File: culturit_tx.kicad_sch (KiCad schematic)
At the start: 0 parts

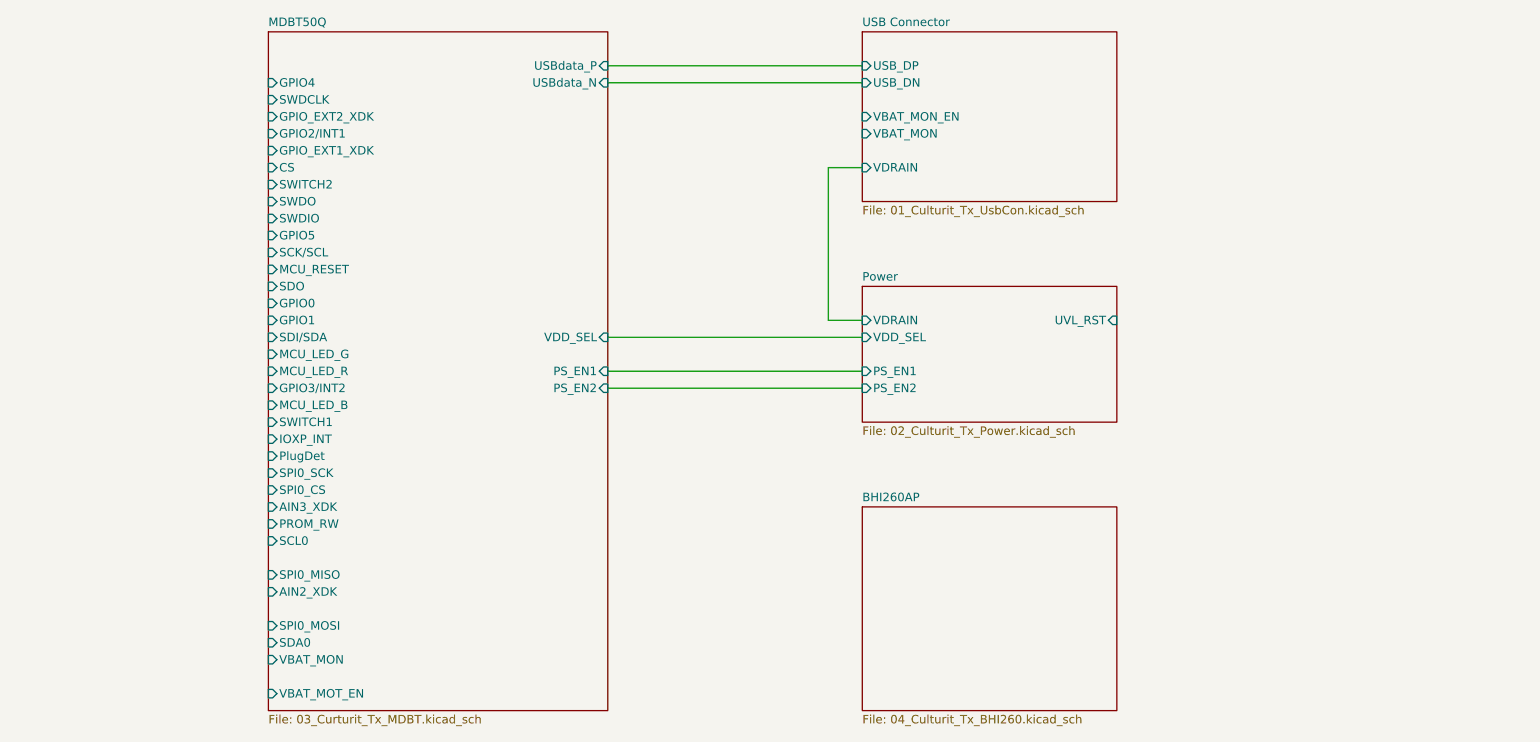
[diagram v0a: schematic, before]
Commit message: 2022-08-10
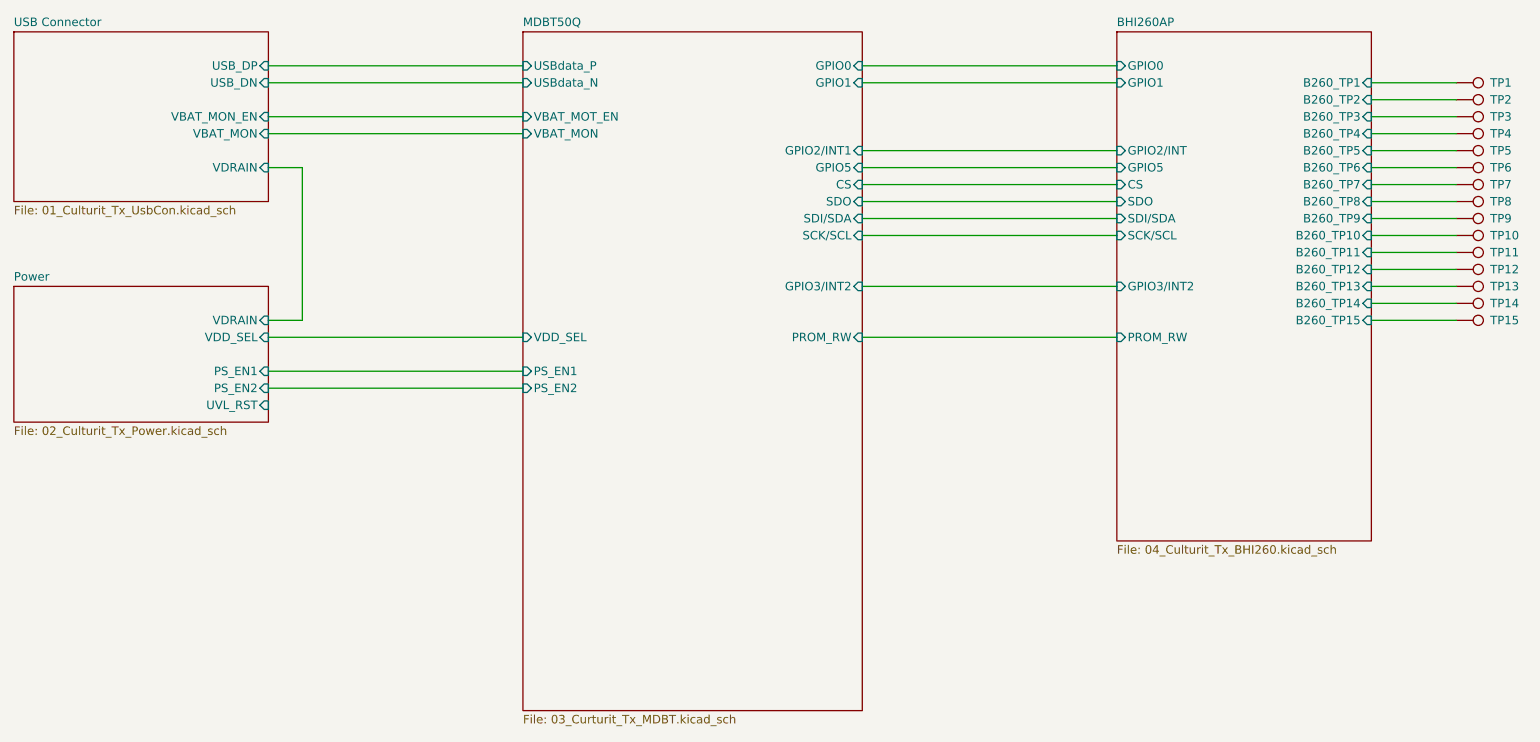
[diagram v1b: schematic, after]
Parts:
- added TP1, TP10, TP11, TP12, TP14, TP15, TP2, TP3, TP4, TP5, TP9: TestPoint, TestPoint:TestPoint_Pad_D2.5mm, symbol Connector:TestPoint
- added TP13, TP6, TP7, TP8: TestPoint, TestPoint:TestPoint_Pad_D4.0mm, symbol Connector:TestPoint
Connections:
- new net BHI260AP/B260_TP1: TP1.1
- new net BHI260AP/B260_TP10: TP10.1
- new net BHI260AP/B260_TP11: TP11.1
- new net BHI260AP/B260_TP12: TP12.1
- new net BHI260AP/B260_TP13: TP13.1
- new net BHI260AP/B260_TP14: TP14.1
- new net BHI260AP/B260_TP15: TP15.1
- new net BHI260AP/B260_TP2: TP2.1
- new net BHI260AP/B260_TP3: TP3.1
- new net BHI260AP/B260_TP4: TP4.1
- new net BHI260AP/B260_TP5: TP5.1
- new net BHI260AP/B260_TP6: TP6.1
- new net BHI260AP/B260_TP7: TP7.1
- new net BHI260AP/B260_TP8: TP8.1
- new net BHI260AP/B260_TP9: TP9.1
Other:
- sheet BHI260AP ports: added B260_TP1, B260_TP10, B260_TP11, B260_TP12, B260_TP13, B260_TP14, B260_TP15, B260_TP2, B260_TP3, B260_TP4, B260_TP5, B260_TP6, B260_TP7, B260_TP8, B260_TP9, CS, GPIO0, GPIO1, GPIO2/INT, GPIO3/INT2, GPIO5, PROM_RW, SCK/SCL, SDI/SDA, SDO; removed none
- sheet MDBT50Q ports: added none; removed AIN2_XDK, AIN3_XDK, GPIO4, GPIO_EXT1_XDK, GPIO_EXT2_XDK, IOXP_INT, MCU_LED_B, MCU_LED_G, MCU_LED_R, MCU_RESET, PlugDet, SCL0, SDA0, SPI0_CS, SPI0_MISO, SPI0_MOSI, SPI0_SCK, SWDCLK, SWDIO, SWDO, SWITCH1, SWITCH2
